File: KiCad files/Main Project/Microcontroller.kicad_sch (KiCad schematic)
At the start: 11 parts, among them J1 USBasp, SW1 SW_Push, U18 ATmega328-A, Y1 16MHz

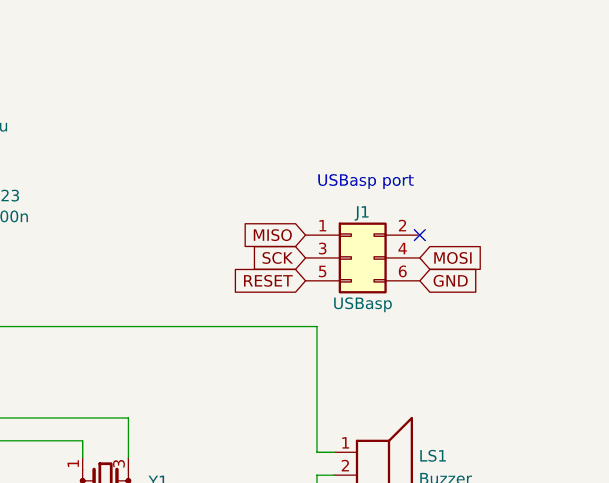
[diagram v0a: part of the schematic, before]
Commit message: update
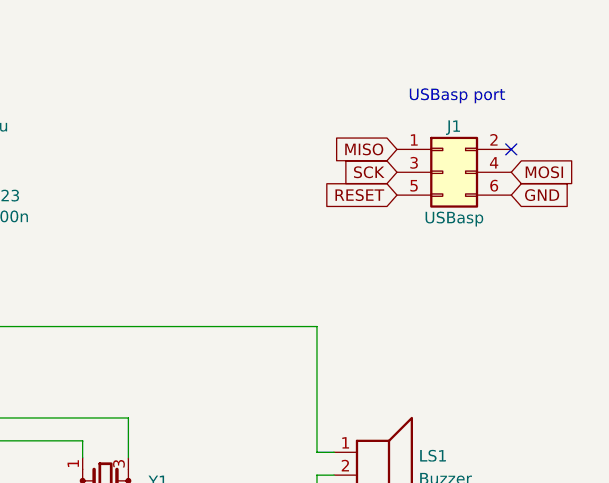
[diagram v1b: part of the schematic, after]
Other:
- moved on the sheet: J1
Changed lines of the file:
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@@
   (no_connect (at 153.67 63.5))
   (no_connect (at 123.19 71.12))
-  (no_connect (at 210.185 58.42))
+  (no_connect (at 220.345 48.895))
   (no_connect (at 153.67 86.36))
   (no_connect (at 153.67 88.9))
@@
     (stroke (width 0) (type default) (color 0 0 0 0))
   )
-  (text "USBasp port" (at 198.755 53.34 0)
+  (text "USBasp port" (at 208.915 43.815 0)
     (effects (font (size 1.27 1.27)) (justify left bottom))
   )
-  (global_label "MISO" (shape input) (at 197.485 58.42 180) (fields_autoplaced)
+  (global_label "MISO" (shape input) (at 207.645 48.895 180) (fields_autoplaced)
     (effects (font (size 1.27 1.27)) (justify right))
-    (property "Intersheet References" "${INTERSHEET_REFS}" (id 0) (at -27.94 3.175 0)
+    (property "Intersheet References" "${INTERSHEET_REFS}" (id 0) (at -17.78 -6.35 0)
       (effects (font (size 1.27 1.27)) hide)
     )
@@
     )
   )
-  (global_label "GND" (shape input) (at 210.185 63.5 0) (fields_autoplaced)
-    (effects (font (size 1.27 1.27)) (justify left))
-    (property "Intersheet References" "${INTERSHEET_REFS}" (id 0) (at -27.94 3.175 0)
-      (effects (font (size 1.27 1.27)) hide)
-    )
-  )
-  (global_label "RESET" (shape input) (at 197.485 63.5 180) (fields_autoplaced)
+  (global_label "GND" (shape input) (at 220.345 53.975 0) (fields_autoplaced)
+    (effects (font (size 1.27 1.27)) (justify left))
+    (property "Intersheet References" "${INTERSHEET_REFS}" (id 0) (at -17.78 -6.35 0)
+      (effects (font (size 1.27 1.27)) hide)
+    )
+  )
+  (global_label "RESET" (shape input) (at 207.645 53.975 180) (fields_autoplaced)
     (effects (font (size 1.27 1.27)) (justify right))
-    (property "Intersheet References" "${INTERSHEET_REFS}" (id 0) (at -27.94 3.175 0)
+    (property "Intersheet References" "${INTERSHEET_REFS}" (id 0) (at -17.78 -6.35 0)
       (effects (font (size 1.27 1.27)) hide)
     )
@@
     )
   )
-  (global_label "MOSI" (shape input) (at 210.185 60.96 0) (fields_autoplaced)
-    (effects (font (size 1.27 1.27)) (justify left))
-    (property "Intersheet References" "${INTERSHEET_REFS}" (id 0) (at -27.94 3.175 0)
+  (global_label "MOSI" (shape input) (at 220.345 51.435 0) (fields_autoplaced)
+    (effects (font (size 1.27 1.27)) (justify left))
+    (property "Intersheet References" "${INTERSHEET_REFS}" (id 0) (at -17.78 -6.35 0)
       (effects (font (size 1.27 1.27)) hide)
     )
@@
     )
   )
-  (global_label "SCK" (shape input) (at 197.485 60.96 180) (fields_autoplaced)
+  (global_label "SCK" (shape input) (at 207.645 51.435 180) (fields_autoplaced)
     (effects (font (size 1.27 1.27)) (justify right))
-    (property "Intersheet References" "${INTERSHEET_REFS}" (id 0) (at -27.94 3.175 0)
+    (property "Intersheet References" "${INTERSHEET_REFS}" (id 0) (at -17.78 -6.35 0)
       (effects (font (size 1.27 1.27)) hide)
     )
@@
     (pin "1")
   )
-  (symbol (lib_id "Connector_Generic:Conn_02x03_Odd_Even") (at 202.565 60.96 0) (unit 1)
-    (in_bom yes) (on_board yes)
-    (property "Reference" "J1" (id 0) (at 203.835 55.88 0))
-    (property "Value" "USBasp" (id 1) (at 203.835 66.04 0))
-    (property "Footprint" "Connector_PinSocket_1.27mm:PinSocket_2x03_P1.27mm_Vertical" (id 2) (at 202.565 60.96 0)
-      (effects (font (size 1.27 1.27)) hide)
-    )
-    (property "Datasheet" "~" (id 3) (at 202.565 60.96 0)
-      (effects (font (size 1.27 1.27)) hide)
-    )
-    (property "Basic/Extended" "-" (id 4) (at 202.565 60.96 0)
-      (effects (font (size 1.27 1.27)) hide)
-    )
-    (property "JLCPCB Part #" "-" (id 5) (at 202.565 60.96 0)
-      (effects (font (size 1.27 1.27)) hide)
-    )
-    (property "U labosu?" "Da" (id 6) (at 202.565 60.96 0)
-      (effects (font (size 1.27 1.27)) hide)
-    )
+  (symbol (lib_id "Connector_Generic:Conn_02x03_Odd_Even") (at 212.725 51.435 0) (unit 1)
+    (in_bom yes) (on_board yes)
+    (property "Reference" "J1" (id 0) (at 213.995 46.355 0))
+    (property "Value" "USBasp" (id 1) (at 213.995 56.515 0))
+    (property "Footprint" "Connector_PinSocket_1.27mm:PinSocket_2x03_P1.27mm_Vertical" (id 2) (at 212.725 51.435 0)
+      (effects (font (size 1.27 1.27)) hide)
+    )
+    (property "Datasheet" "~" (id 3) (at 212.725 51.435 0)
+      (effects (font (size 1.27 1.27)) hide)
+    )
+    (property "Basic/Extended" "-" (id 4) (at 212.725 51.435 0)
+      (effects (font (size 1.27 1.27)) hide)
+    )
+    (property "JLCPCB Part #" "-" (id 5) (at 212.725 51.435 0)
+      (effects (font (size 1.27 1.27)) hide)
+    )
+    (property "U labosu?" "Da" (id 6) (at 212.725 51.435 0)
+      (effects (font (size 1.27 1.27)) hide)
+    )
